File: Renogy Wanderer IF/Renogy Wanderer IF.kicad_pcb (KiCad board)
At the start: 2 copper layers, 50.8 x 40.6 mm, 4 parts, among them J1 Conn_01x04, U1 WeMos_D1_mini

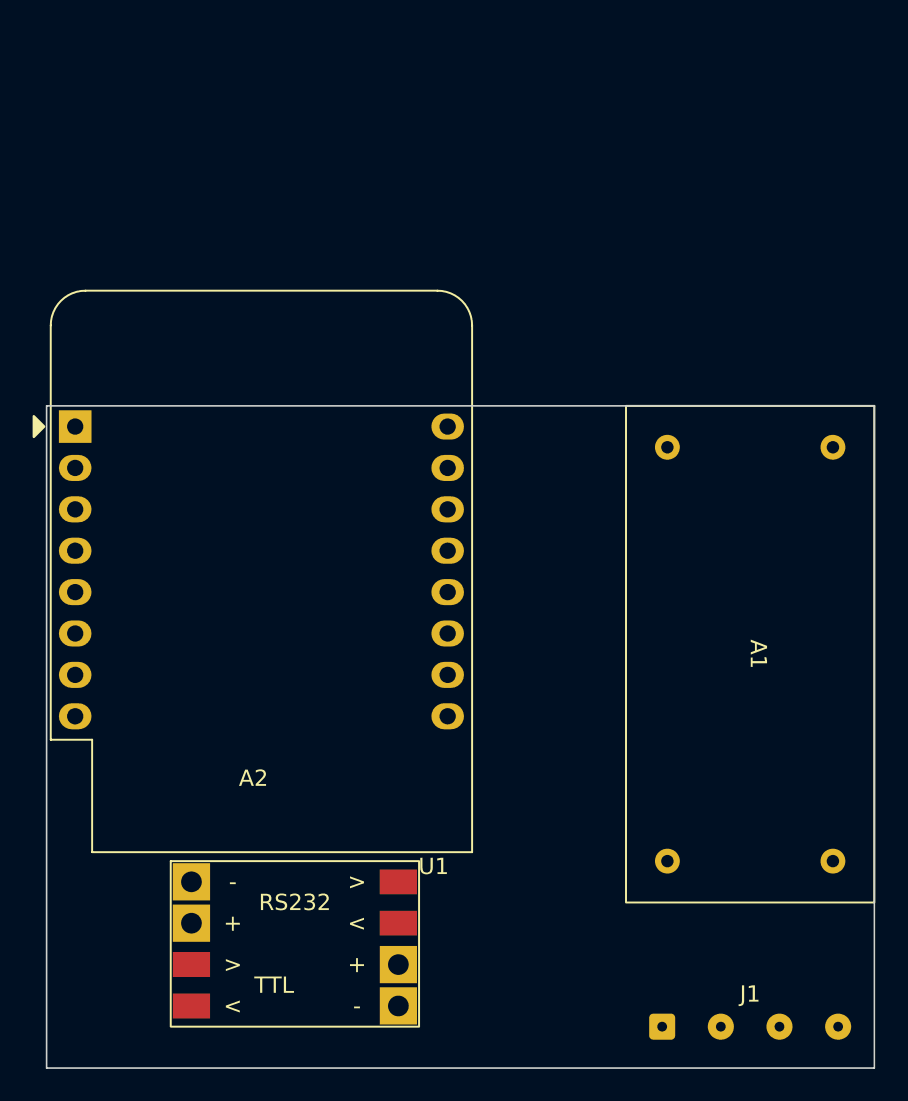
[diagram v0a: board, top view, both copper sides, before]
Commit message: Initial PCB design
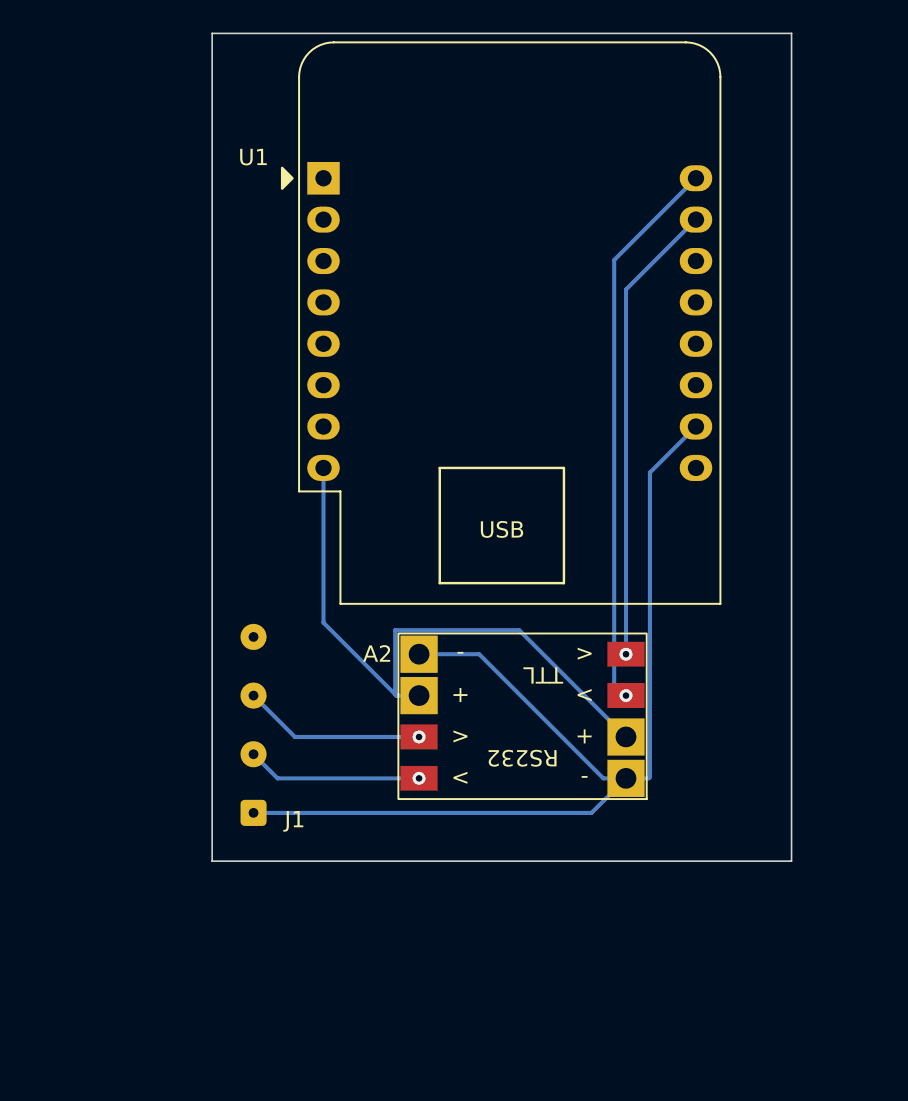
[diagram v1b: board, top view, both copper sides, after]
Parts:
- removed A1: MINI-360, Module:MINI-360
- moved J1 28.3 mm to (99.1, 91.0), turned to 90 degrees
- moved U1 21.6 mm to (103.4, 52.1)
- moved A2 18.0 mm to (114.3, 86.4), turned to 180 degrees
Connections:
- J1 pad 1: +15V -> GND
- J1 pad 4: GND -> unconnected-(J1-Pad4)
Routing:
- net GND: track 0.00 -> 63.8 mm
- net +3V3: track 0.00 -> 38.1 mm
- net Net-(U1-Pad16): track 0.00 -> 34.1 mm, vias 0 -> 1
- net Net-(U1-Pad15): track 0.00 -> 28.4 mm, vias 0 -> 1
- net Net-(J1-Pad3): track 0.00 -> 11.2 mm, vias 0 -> 1
- net Net-(J1-Pad2): track 0.00 -> 10.8 mm, vias 0 -> 1
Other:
- board size 50.8 x 40.6 mm -> 35.6 x 50.8 mm
- board text added: "USB"
